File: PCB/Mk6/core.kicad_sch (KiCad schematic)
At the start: 12 parts, among them J2 Bank, J25 Debug, U3 GAL20V8B-10, U4 R65C02, U5 EEPROM, U8 62256

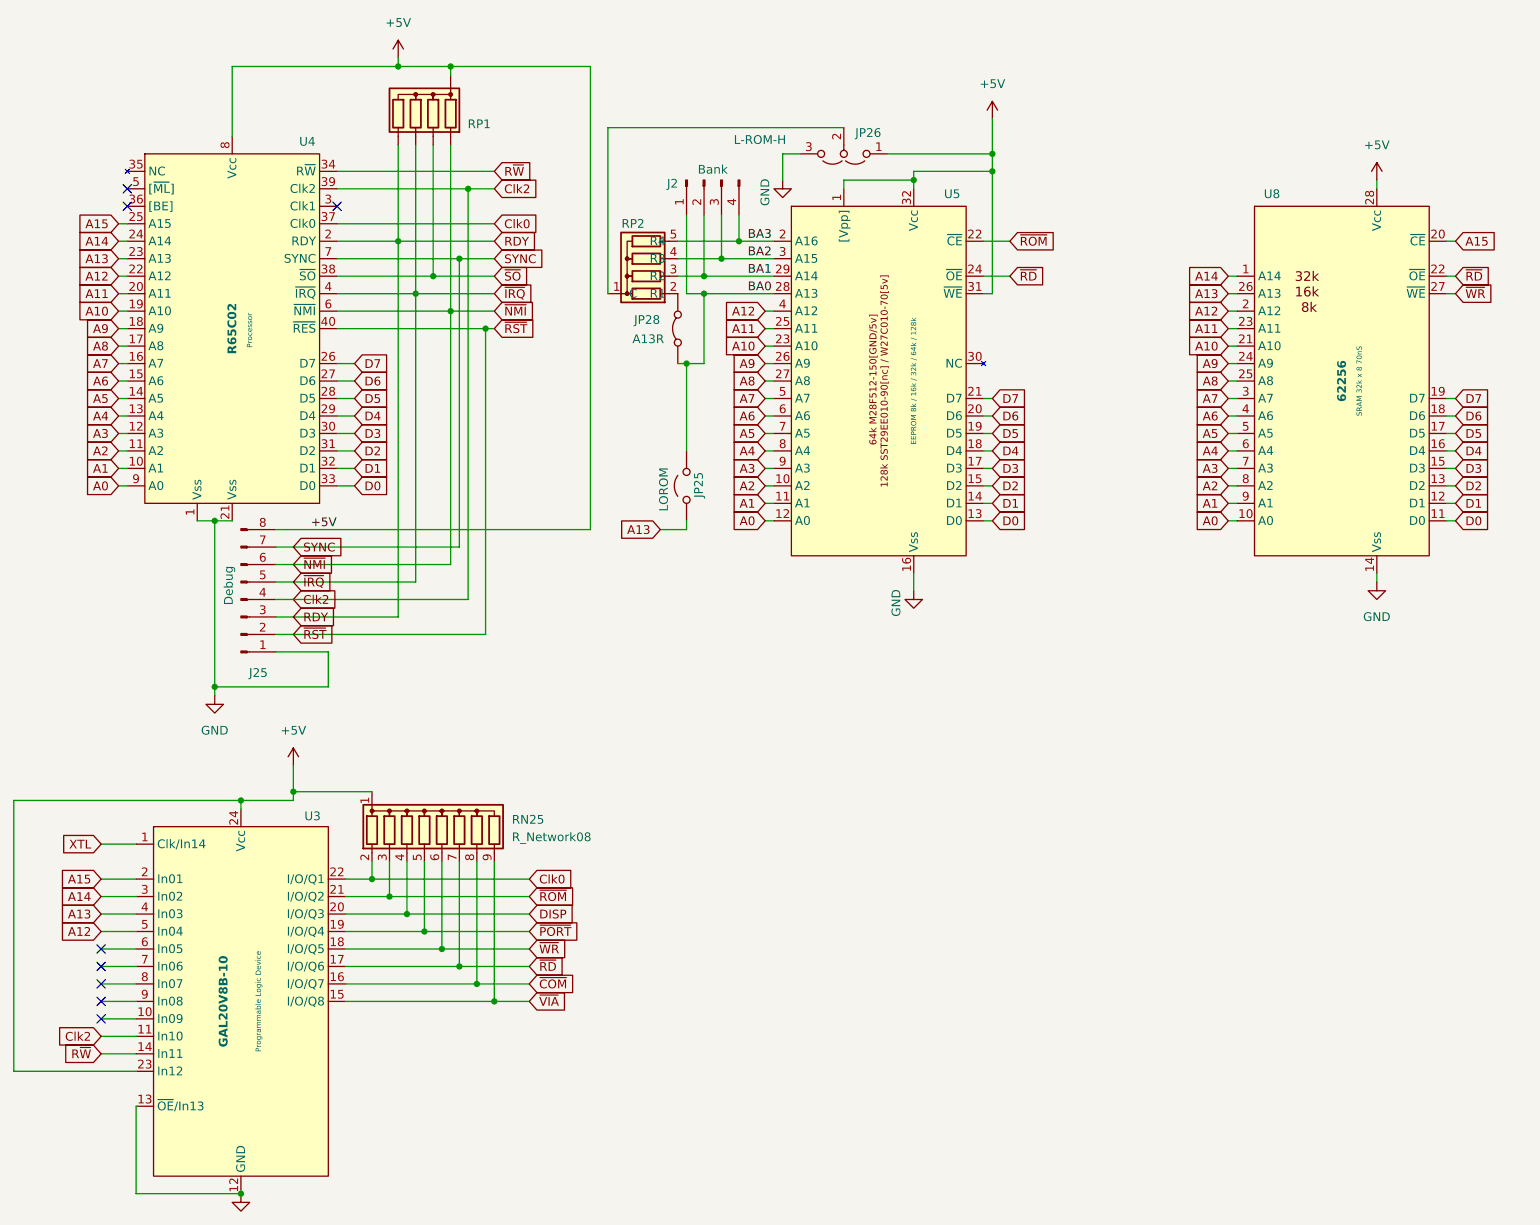
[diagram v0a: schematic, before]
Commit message: save point
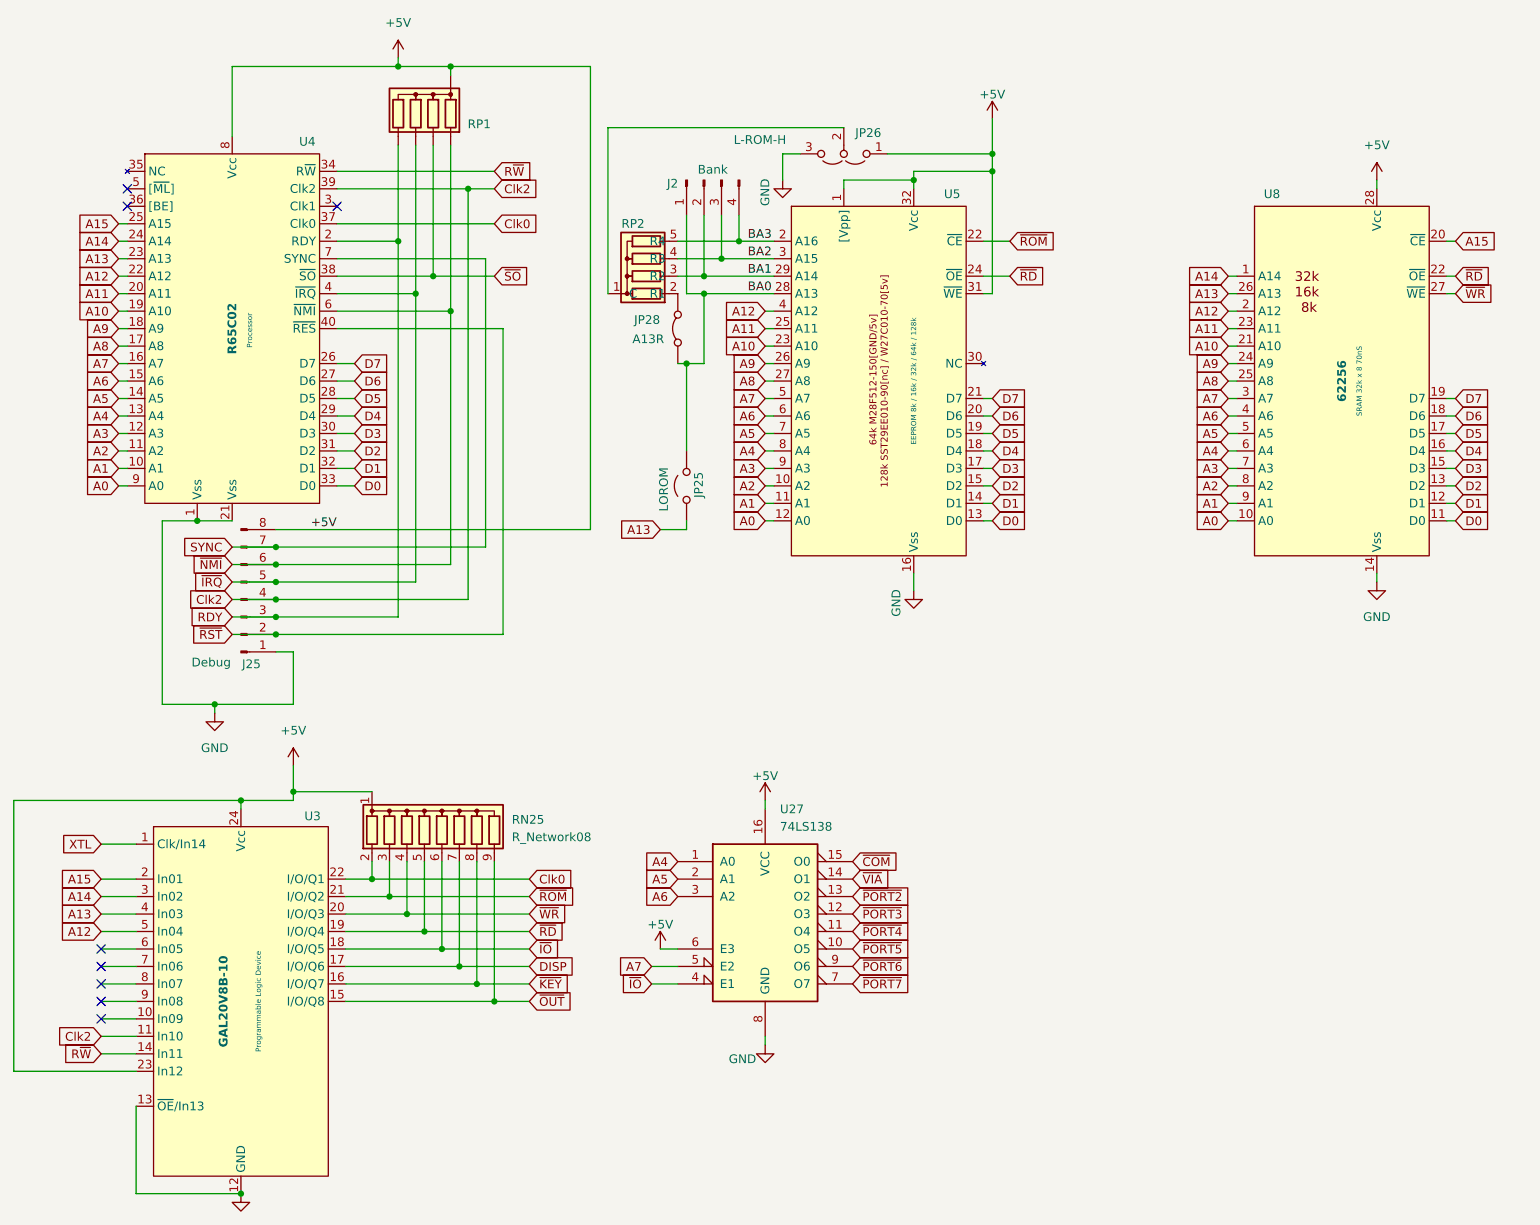
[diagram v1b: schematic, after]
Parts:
- added U27: 74LS138, symbol 74xx:74LS138
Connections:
- net ~{PORT} is gone; now on net ~{RD}: RN25.5 (R4), U3.19 (I/O/Q4)
- net +5V: now also U27.16 (VCC), U27.6 (E3)
- net A4: now also U27.1 (A0)
- net A5: now also U27.2 (A1)
- net A6: now also U27.3 (A2)
- net A7: now also U27.5 (E2)
- net DISP: now also RN25.7 (R6), U3.17 (I/O/Q6); no longer RN25.4 (R3), U3.20 (I/O/Q3)
- net GND: now also U27.8 (GND)
- net ~{COM}: now also U27.15 (O0); no longer RN25.8 (R7), U3.16 (I/O/Q7)
- net ~{RD}: no longer RN25.7 (R6), U3.17 (I/O/Q6)
- net ~{VIA}: now also U27.14 (O1); no longer RN25.9 (R8), U3.15 (I/O/Q8)
- net ~{WR}: now also RN25.4 (R3), U3.20 (I/O/Q3); no longer RN25.6 (R5), U3.18 (I/O/Q5)
- new net ~{IO}: RN25.6 (R5), U27.4 (E1), U3.18 (I/O/Q5)
- new net ~{KEY}: RN25.8 (R7), U3.16 (I/O/Q7)
- new net ~{OUT}: RN25.9 (R8), U3.15 (I/O/Q8)
- new net ~{PORT2}: U27.13 (O2)
- new net ~{PORT3}: U27.12 (O3)
- new net ~{PORT4}: U27.11 (O4)
- new net ~{PORT5}: U27.10 (O5)
- new net ~{PORT6}: U27.9 (O6)
- new net ~{PORT7}: U27.7 (O7)
